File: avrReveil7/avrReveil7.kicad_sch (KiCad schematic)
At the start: 3 parts, among them J1 Conn_01x06, J2 Conn_01x06, U1 TM1637 (generic clockwise SOP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

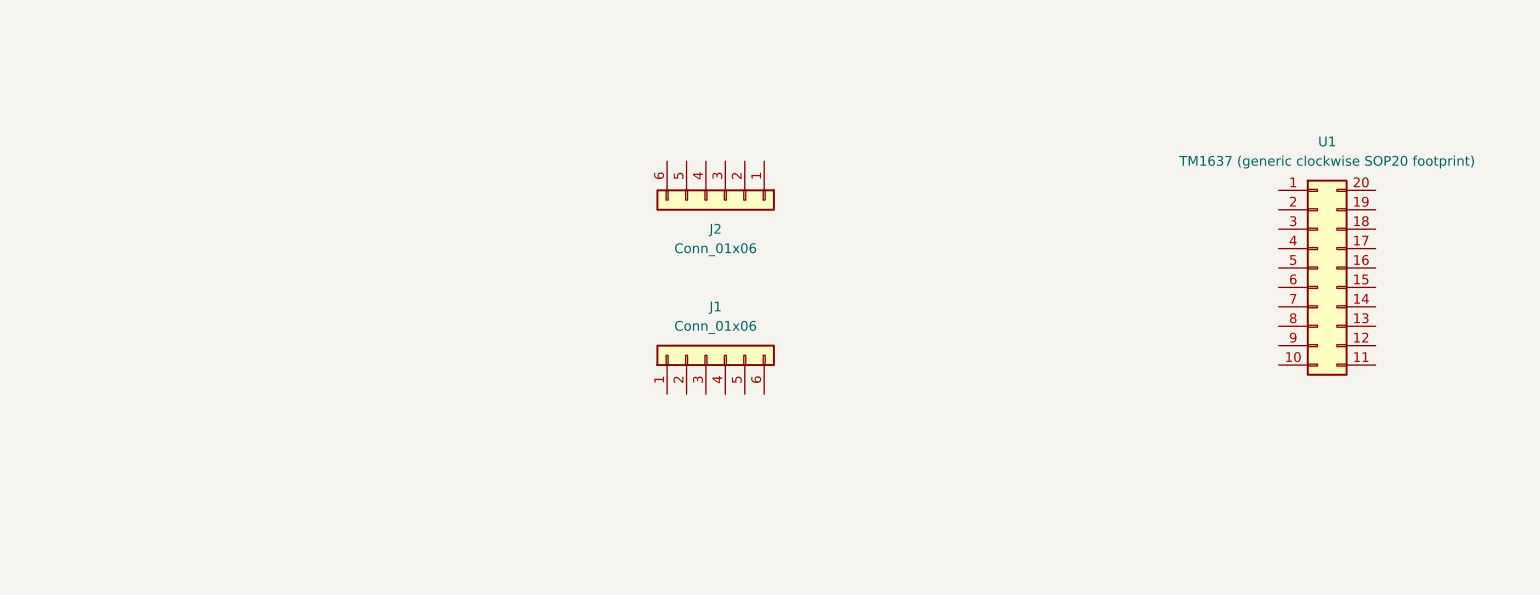
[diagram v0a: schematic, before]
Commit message: avrReveil7 initial commit
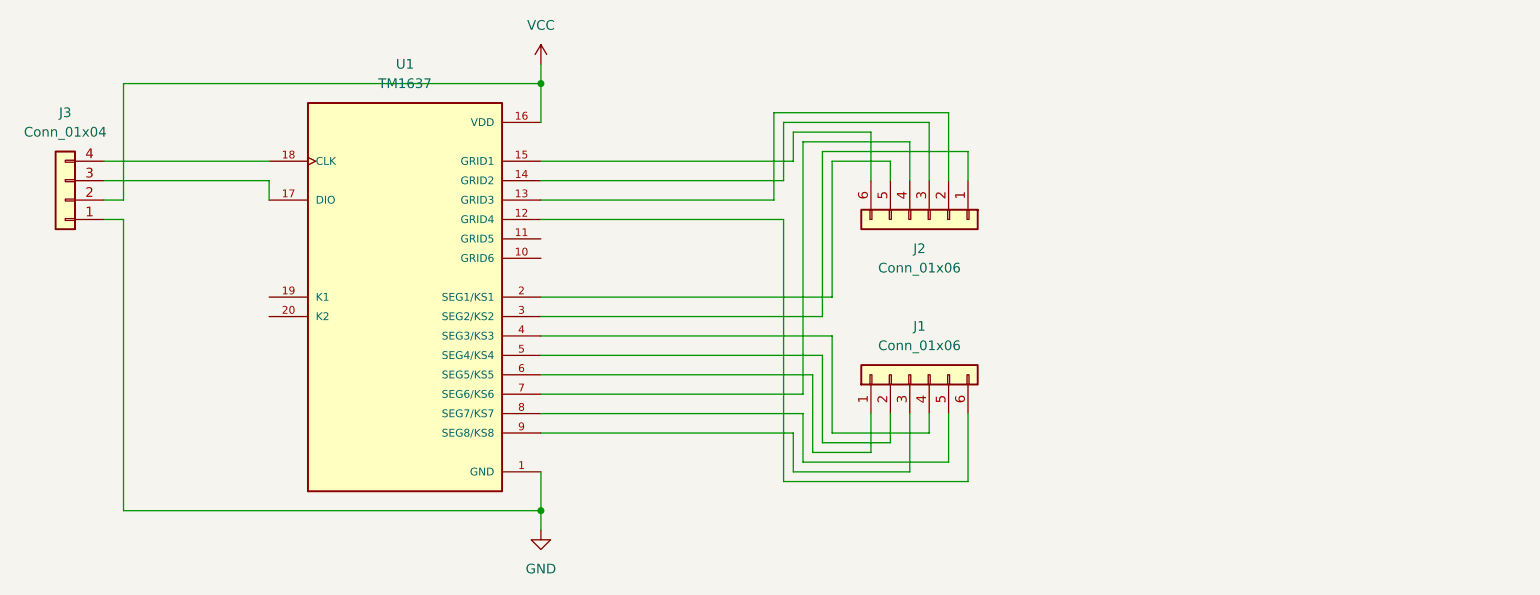
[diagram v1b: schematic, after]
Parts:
- removed U1: TM1637 (generic clockwise SOP20 footprint), Connector_Wuerth:Wuerth_WR-PHD_613020216921_Large_2x10_P2.54mm_Vertical, symbol Connector_Generic:Conn_02x10_Counter_Clockwise
- added J3: Conn_01x04, Connector_PinSocket_2.54mm:PinSocket_1x04_P2.54mm_Vertical, symbol Sparkfun conn:Conn_01x04
- added U1: TM1637, Package_DIP:DIP-20_W7.62mm, symbol TM1637:TM1637
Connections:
- net at J2.1 (Pin_1): now also U1.3 (SEG2/KS2)
- net at J2.2 (Pin_2): now also U1.13 (GRID3)
- net at J2.3 (Pin_3): now also U1.14 (GRID2)
- net at J2.4 (Pin_4): now also U1.7 (SEG6/KS6)
- net at J2.5 (Pin_5): now also U1.2 (SEG1/KS1)
- net at J2.6 (Pin_6): now also U1.15 (GRID1)
- net at J1.1 (Pin_1): now also U1.6 (SEG5/KS5)
- net at J1.2 (Pin_2): now also U1.5 (SEG4/KS4)
- net at J1.3 (Pin_3): now also U1.9 (SEG8/KS8)
- net at J1.4 (Pin_4): now also U1.4 (SEG3/KS3)
- net at J1.5 (Pin_5): now also U1.8 (SEG7/KS7)
- net at J1.6 (Pin_6): now also U1.12 (GRID4)
- new net: J3.3 (Pin_3), U1.17 (DIO)
- new net: J3.4 (Pin_4), U1.18 (CLK)
- new net GND: J3.1 (Pin_1), U1.1 (GND)
- new net VCC: J3.2 (Pin_2), U1.16 (VDD)
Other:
- moved on the sheet: J1, J2
